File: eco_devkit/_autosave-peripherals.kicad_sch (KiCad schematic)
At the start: 24 parts, among them J2 BluetoothHeader, J3 Buttons, J4 J_MOSFET, J5 LEDS, Q1 MOSFET, Q2 2N2219, SW3 PTS636, SW4 PTS636, SW5 PTS636, SW6 PTS636

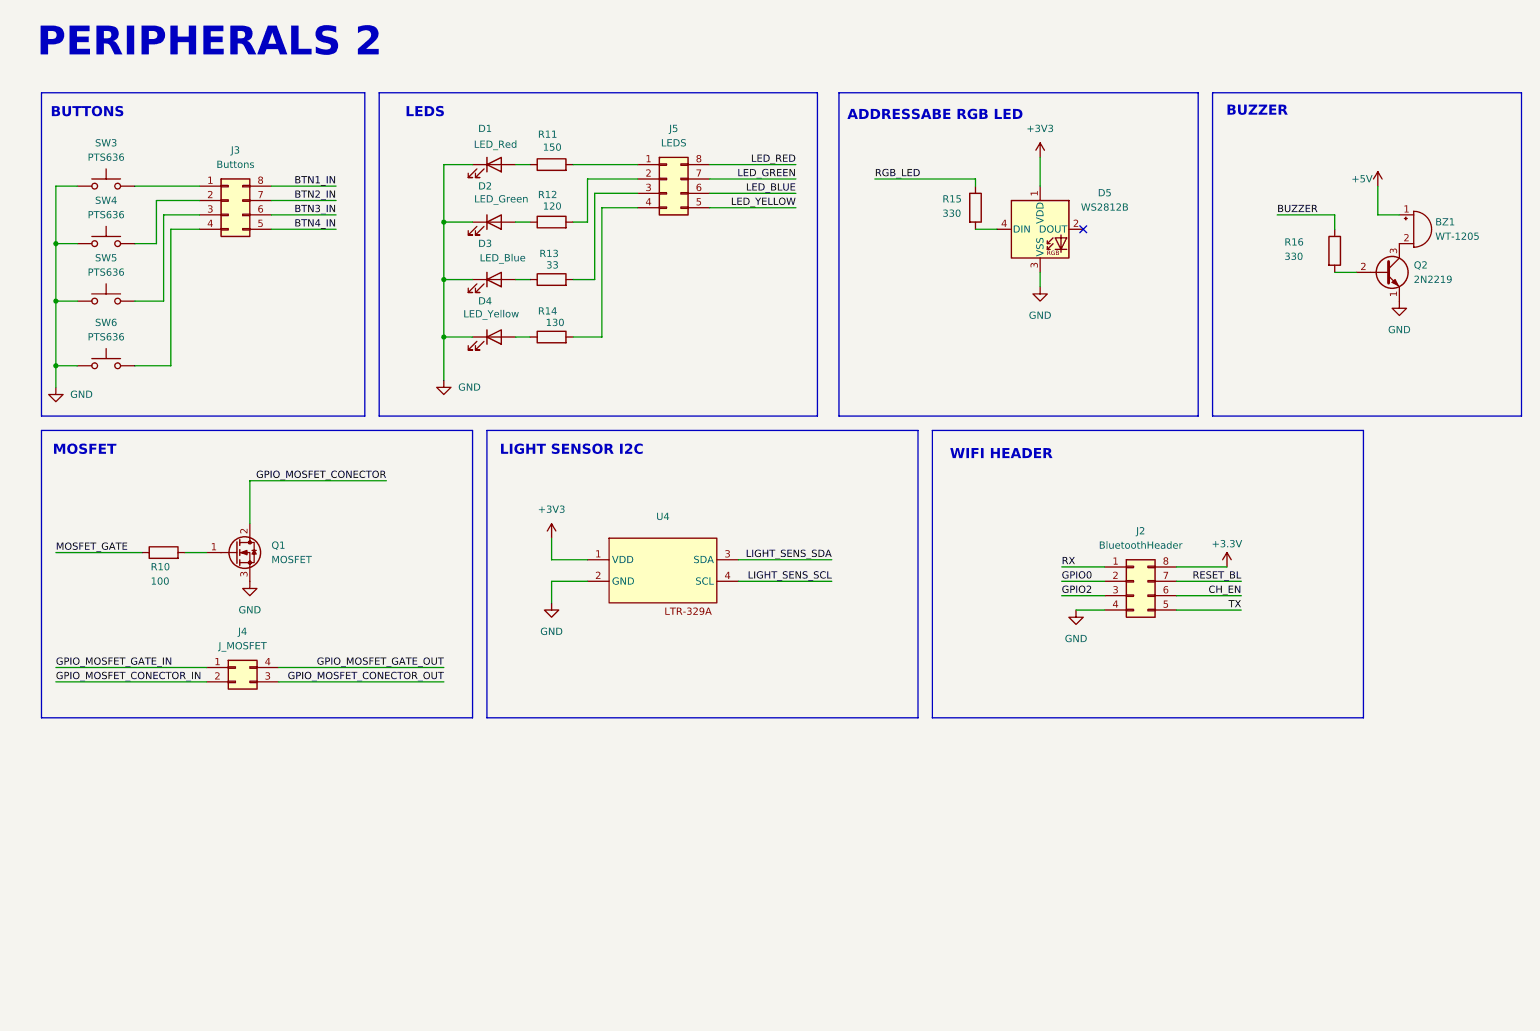
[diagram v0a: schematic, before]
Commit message: chore: ajustes nos periféricos
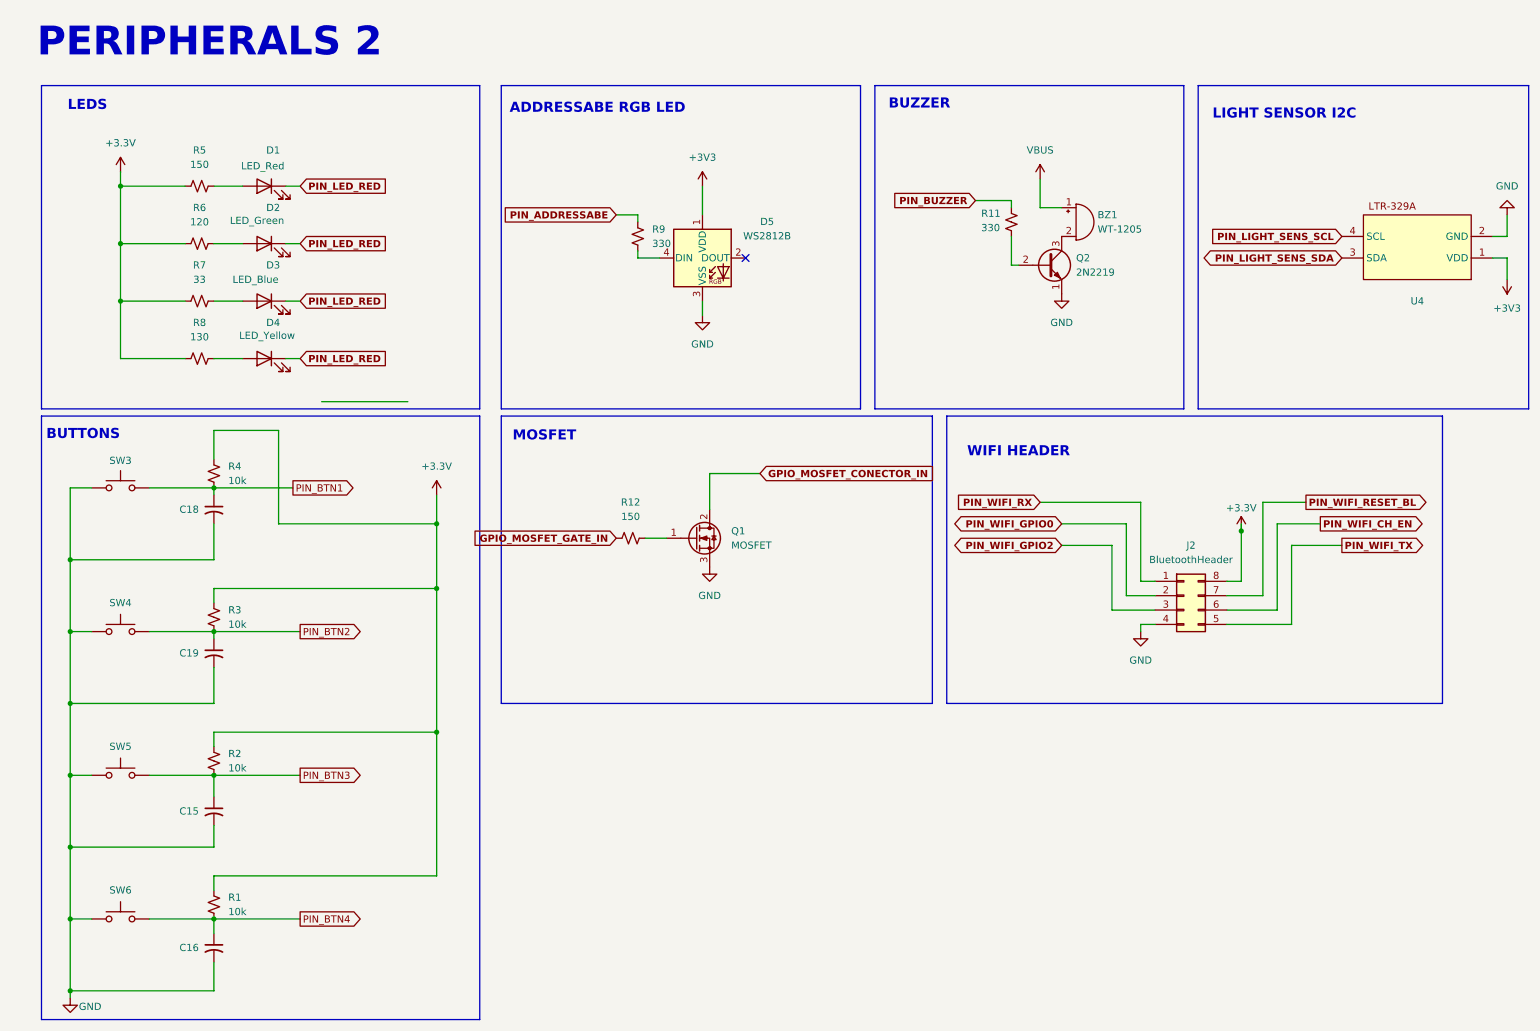
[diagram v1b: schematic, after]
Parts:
- removed J3: Buttons, Connector_PinHeader_2.54mm:PinHeader_2x04_P2.54mm_Vertical, symbol Connector_Generic:Conn_02x04_Counter_Clockwise
- removed J4: J_MOSFET, symbol Connector_Generic:Conn_02x02_Counter_Clockwise
- removed J5: LEDS, Connector_PinHeader_2.54mm:PinHeader_2x04_P2.54mm_Vertical, symbol Connector_Generic:Conn_02x04_Counter_Clockwise
- removed R10: 100, Resistor_SMD:R_0402_1005Metric, symbol Device:R
- removed R11: 150, Resistor_SMD:R_0402_1005Metric, symbol Device:R
- removed R12: 120, Resistor_SMD:R_0402_1005Metric, symbol Device:R
- removed R13: 33, Resistor_SMD:R_0402_1005Metric, symbol Device:R
- removed R14: 130, Resistor_SMD:R_0402_1005Metric, symbol Device:R
- removed R15, R16: 330, Resistor_SMD:R_0402_1005Metric, symbol Device:R
- added C15, C16, C18, C19: C_Small_US, symbol Device:C_Small_US
- added R1, R2, R3, R4: 10k, symbol Device:R_Small_US
- added R11, R9: 330, symbol Device:R_Small_US
- added R12, R5: 150, symbol Device:R_Small_US
- added R6: 120, symbol Device:R_Small_US
- added R7: 33, symbol Device:R_Small_US
- added R8: 130, symbol Device:R_Small_US
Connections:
- net GPIO_MOSFET_CONECTOR is gone; now on net GPIO_MOSFET_CONECTOR_IN: Q1.2 (D)
- net +3.3V: now also R1.1, R2.1, R3.1, R4.1, R5.2, R6.2, R7.2, R8.2
- net GND: now also C15.2, C16.2, C18.2, C19.2; no longer D1.1 (K), D2.1 (K), D3.1 (K), D4.1 (K)
- net GPIO_MOSFET_GATE_IN: now also R12.2
- net at D3.2 (A): now also R7.1
- net at D2.2 (A): now also R6.1
- net at D4.2 (A): now also R8.1
- net PIN_BTN1: now reaches SW3.2
- net PIN_BTN1: now also C18.1, R4.2
- net PIN_BTN2: now reaches SW4.2
- net PIN_BTN2: now also C19.1, R3.2
- net PIN_BTN3: now reaches SW5.2
- net PIN_BTN3: now also C15.1, R2.2
- net PIN_BTN4: now reaches SW6.2
- net PIN_BTN4: now also C16.1, R1.2
- net at Q1.1 (G): now also R12.1
- net at D1.2 (A): now also R5.1
- net at Q2.2 (B): now also R11.2
- net at D5.4 (DIN): now also R9.2
- net +5V renamed VBUS
- net CH_EN renamed PIN_WIFI_CH_EN
- net GPIO0 renamed PIN_WIFI_GPIO0
- net GPIO2 renamed PIN_WIFI_GPIO2
- net LIGHT_SENS_SCL renamed PIN_LIGHT_SENS_SCL
- net LIGHT_SENS_SDA renamed PIN_LIGHT_SENS_SDA
- net RESET_BL renamed PIN_WIFI_RESET_BL
- net RX renamed PIN_WIFI_RX
- net TX renamed PIN_WIFI_TX
- new net PIN_ADDRESSABE: R9.1
- new net PIN_BUZZER: R11.1
- new net PIN_LED_RED: D1.1 (K), D2.1 (K), D3.1 (K), D4.1 (K)
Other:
- moved on the sheet: BZ1, D1, D2, D3, D4, D5, J2, Q1, Q2, SW3, SW4, SW5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
